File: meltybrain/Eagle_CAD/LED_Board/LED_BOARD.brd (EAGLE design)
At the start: 58 x 10 mm, 17 parts, among them J1 SM04B-SRSS-TB(LF)(SN)

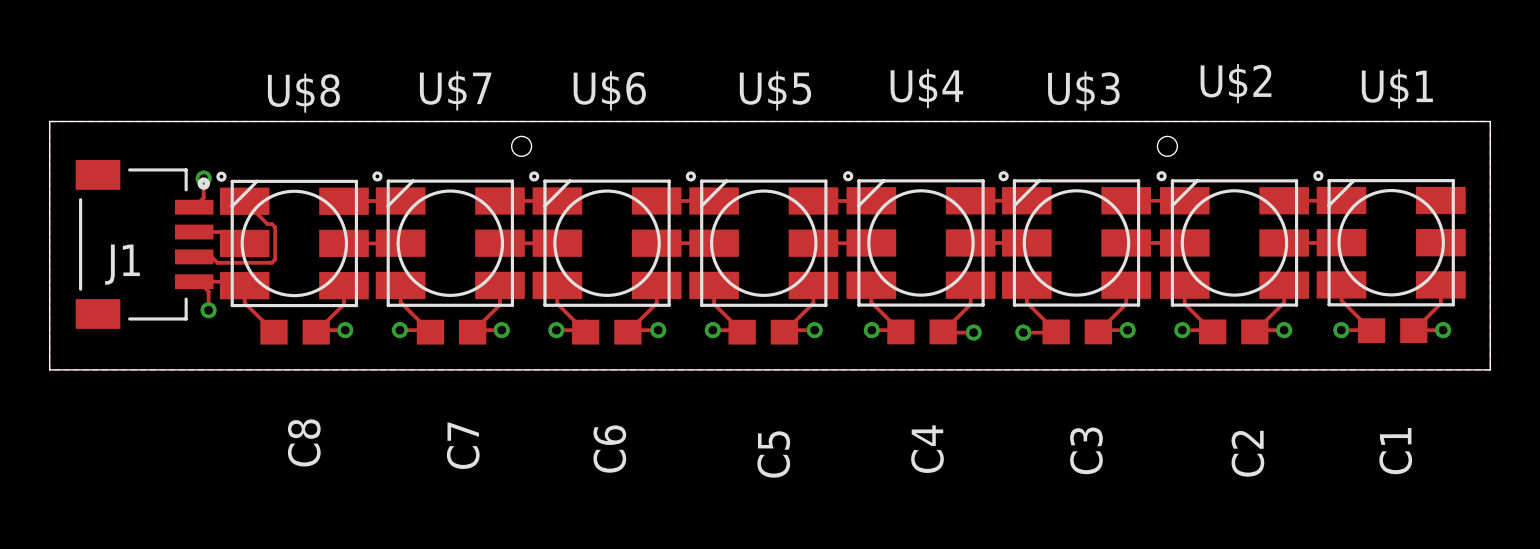
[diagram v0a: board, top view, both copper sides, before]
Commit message: Update LED_BOARD.brd
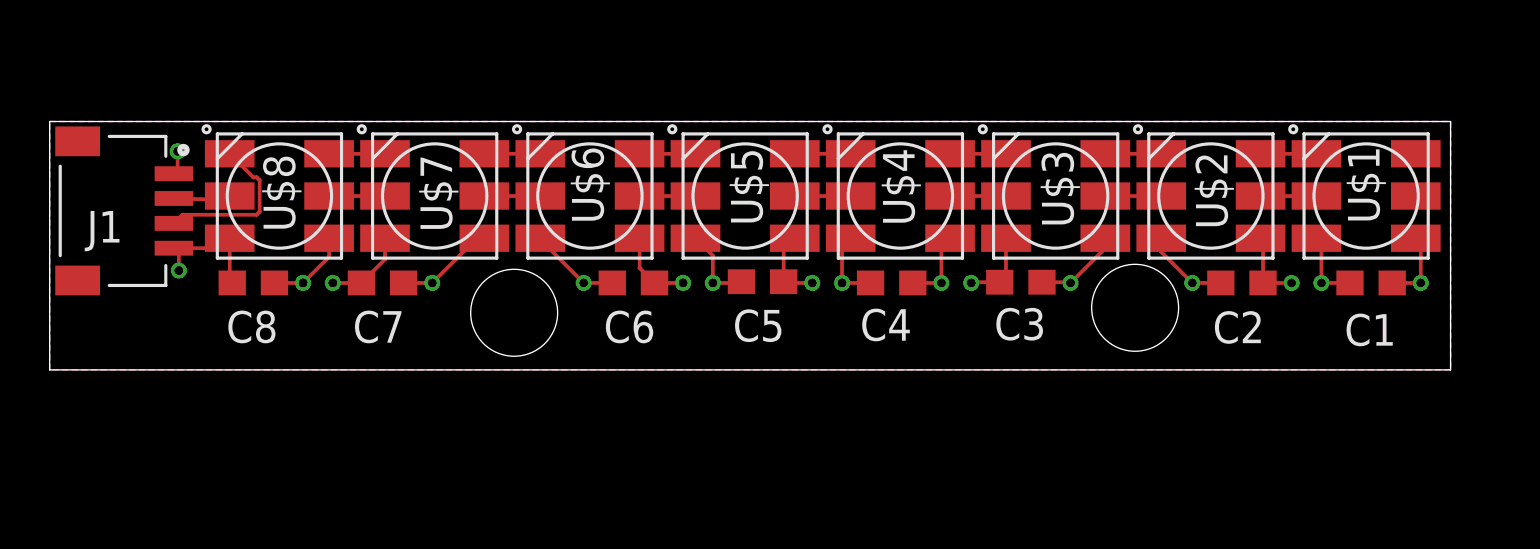
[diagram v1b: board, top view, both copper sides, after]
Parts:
- moved C7 3.41 mm to (13.4, 3.50)
- moved C3 3.03 mm to (39.1, 3.53)
- moved C8 2.60 mm to (8.20, 3.50)
- moved C4 2.32 mm to (33.9, 3.50)
- moved C6 2.25 mm to (23.5, 3.50)
- moved U$1 2.13 mm to (53.0, 7.00)
- moved U$2 2.12 mm to (46.8, 7.00)
- moved C1 2.11 mm to (53.2, 3.50)
- moved U$3 2.07 mm to (40.5, 7.00)
- moved U$4 2.06 mm to (34.2, 7.00)
- moved U$5 2.04 mm to (28.0, 7.00)
- moved C5 2.03 mm to (28.7, 3.55)
- moved U$6 2.02 mm to (21.8, 7.00)
- moved U$8 2.00 mm to (9.25, 7.00)
- moved U$7 2.00 mm to (15.5, 7.00)
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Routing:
- net GND: track 31.4 -> 29.1 mm
- net +5V: track 29.8 -> 28.0 mm
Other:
- board size 58 x 10 mm -> 56.4 x 10 mm
